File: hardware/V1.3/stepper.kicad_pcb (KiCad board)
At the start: 4 copper layers, 40 x 40 mm, 128 parts, among them J101 USB-MINI-B-SMD, J102 DRILL, J103 DRILL, J104 DRILL, J105 DRILL, J401 STACK-UP-HIGH, J402 STACK-DOWN, J403 STACK-UP-HIGH, J404 STACK-DOWN, P201 black, P202 green, P301 CON-SENSOR, P302 CON-SENSOR, Q201 FDS8449, Q202 AO4421, Q203 2N7002, SW101 Reset, SW102 Erase, U101 AT91SAM3SXB, U102 82400152, U201 ZXCT1086, U202 TMC21XX, U501 LD1117, X101 16Mhz

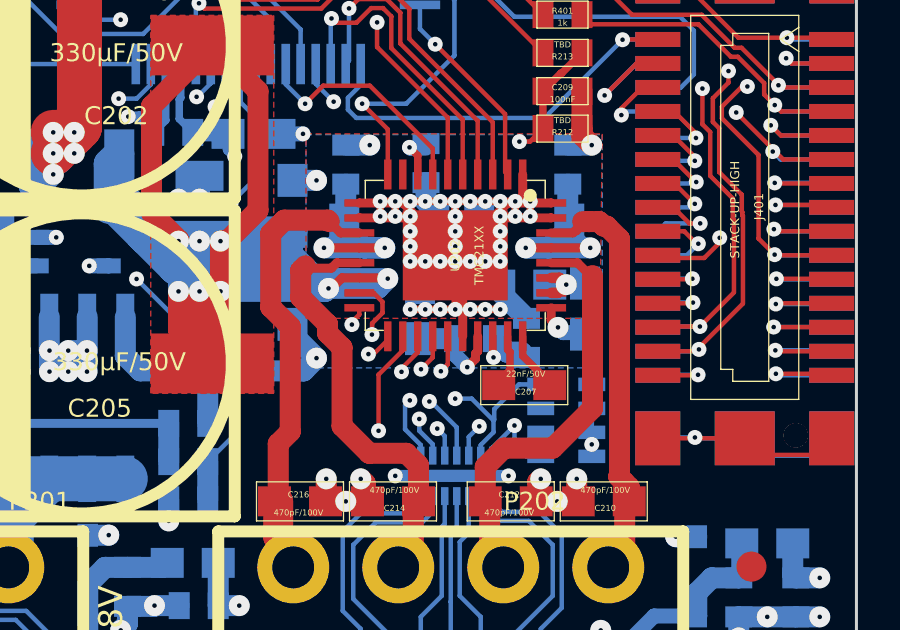
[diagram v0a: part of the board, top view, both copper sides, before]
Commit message: ordered version
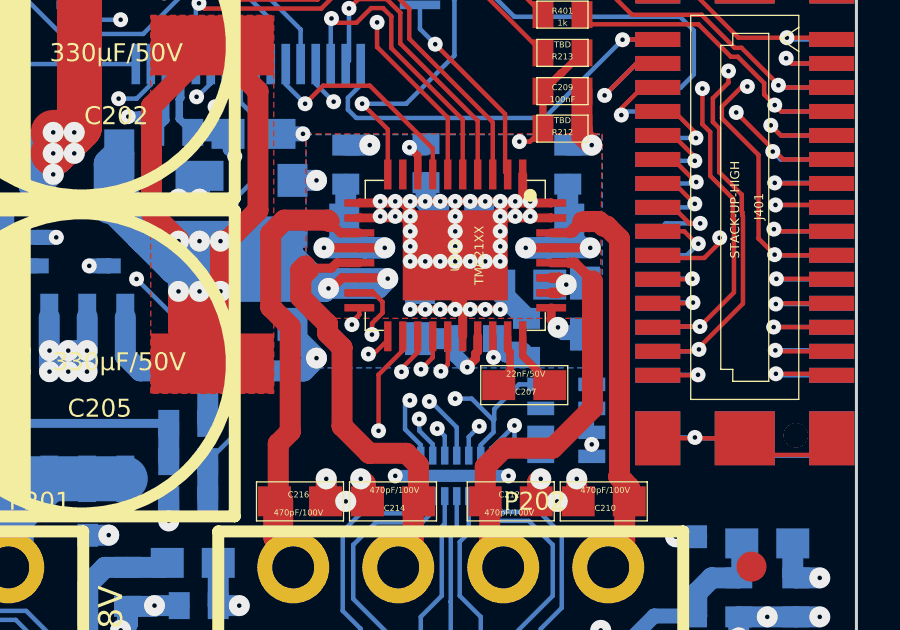
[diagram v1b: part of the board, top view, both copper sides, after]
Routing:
- net M2: track 14.5 -> 15.5 mm
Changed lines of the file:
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@@
     (thickness 1.6002)
     (drawings 64)
-    (tracks 2583)
+    (tracks 2589)
     (zones 0)
     (modules 128)
@@
     (1 GND signal hide)
     (2 VCC signal hide)
-    (31 Rückseite signal hide)
+    (31 Rückseite signal)
     (32 B.Adhes user)
     (33 F.Adhes user)
@@
   )
   (setup
-    (last_trace_width 0.1524)
+    (last_trace_width 0.25)
     (user_trace_width 0.1524)
     (user_trace_width 0.25)
@@
     (pad_to_mask_clearance 0)
     (aux_axis_origin 126.72568 112.776)
-    (visible_elements FFFF5FBF)
+    (visible_elements FFFF9FBF)
     (pcbplotparams
-      (layerselection 0x00030_80000001)
+      (layerselection 0x010f0_80000007)
       (usegerberextensions true)
       (excludeedgelayer true)
       (linewidth 0.150000)
-      (plotframeref true)
+      (plotframeref false)
       (viasonmask false)
       (mode 1)
@@
       (drillshape 0)
       (scaleselection 1)
-      (outputdirectory prod/))
+      (outputdirectory /tmp/stepper/))
   )
   (net 0 "")
@@
   (segment (start 139.15 74.8) (end 139.15 74.3749) (width 0.2998) (layer Rückseite) (net 123))
   (segment (start 139.05 74.6499) (end 139.2 74.8) (width 0.2998) (layer Rückseite) (net 123))
+  (segment (start 157.15 93.6507) (end 157.5257 93.275) (width 0.35) (layer Vorderseite) (net 124))
+  (segment (start 157.6 93.275) (end 157.8 93.275) (width 0.701) (layer Vorderseite) (net 124))
+  (segment (start 157.5257 93.275) (end 157.6 93.275) (width 0.35) (layer Vorderseite) (net 124))
   (segment (start 159.1501 102.6) (end 159.1501 102.1251) (width 0.70104) (layer Vorderseite) (net 124))
   (segment (start 159.1501 102.1251) (end 158.8 101.775) (width 0.70104) (layer Vorderseite) (net 124))
@@
   (segment (start 158.3 93.425) (end 158.3 93.5) (width 0.1524) (layer Vorderseite) (net 124))
   (segment (start 158.3 93.5) (end 158.825 94.025) (width 0.1524) (layer Vorderseite) (net 124))
-  (segment (start 156.54786 93.6507) (end 157.4243 93.6507) (width 0.1524) (layer Vorderseite) (net 124))
-  (segment (start 157.4243 93.6507) (end 157.8 93.275) (width 0.1524) (layer Vorderseite) (net 124))
+  (segment (start 156.54786 93.6507) (end 157.15 93.6507) (width 0.1524) (layer Vorderseite) (net 124))
   (segment (start 158.4 93.425) (end 158.3 93.425) (width 0.701) (layer Vorderseite) (net 124))
   (segment (start 158.15 93.275) (end 157.8 93.275) (width 0.701) (layer Vorderseite) (net 124))
-  (segment (start 157.8 93.275) (end 157.6 93.275) (width 0.701) (layer Vorderseite) (net 124))
   (segment (start 158.3 93.425) (end 158.15 93.275) (width 0.701) (layer Vorderseite) (net 124))
   (segment (start 159 104.25) (end 158.45 104.8) (width 0.701) (layer Vorderseite) (net 124))
@@
   (segment (start 158.4 93.425) (end 158.3 93.425) (width 0.2998) (layer Vorderseite) (net 124))
   (segment (start 158.3 93.425) (end 158.05 93.425) (width 0.2998) (layer Vorderseite) (net 124))
+  (segment (start 157.925 95.25) (end 157.325 94.65) (width 0.35) (layer Vorderseite) (net 125))
+  (segment (start 157.175 94.65) (end 157.175 94.6489) (width 0.35) (layer Vorderseite) (net 125))
+  (segment (start 157.325 94.65) (end 157.175 94.65) (width 0.35) (layer Vorderseite) (net 125))
   (segment (start 154.5 104.35) (end 154.95 104.8) (width 0.701) (layer Vorderseite) (net 125))
   (segment (start 154.5 102.6) (end 154.5 104.35) (width 0.701) (layer Vorderseite) (net 125))
-  (segment (start 157.85 95.075) (end 157.925 95.075) (width 0.2998) (layer Vorderseite) (net 125))
-  (segment (start 157.424 94.6489) (end 157.85 95.075) (width 0.2998) (layer Vorderseite) (net 125))
-  (segment (start 156.548 94.6489) (end 157.424 94.6489) (width 0.2998) (layer Vorderseite) (net 125))
+  (segment (start 156.548 94.6489) (end 157.175 94.6489) (width 0.2998) (layer Vorderseite) (net 125))
   (segment (start 154.35 101.45) (end 154.35 102.425) (width 0.701) (layer Vorderseite) (net 125))
   (segment (start 154.975 100.825) (end 154.35 101.45) (width 0.701) (layer Vorderseite) (net 125))
   (segment (start 156.6 100.825) (end 154.975 100.825) (width 0.701) (layer Vorderseite) (net 125))
   (segment (start 157.925 99.5) (end 156.6 100.825) (width 0.701) (layer Vorderseite) (net 125))
-  (segment (start 157.925 95.075) (end 157.925 99.5) (width 0.701) (layer Vorderseite) (net 125))
+  (segment (start 157.925 95.25) (end 157.925 99.5) (width 0.701) (layer Vorderseite) (net 125))
+  (segment (start 148.2 95.8) (end 148.425 95.575) (width 0.25) (layer Vorderseite) (net 126))
+  (segment (start 148.425 95.225) (end 148.675 94.975) (width 0.25) (layer Vorderseite) (net 126))
+  (segment (start 148.425 95.575) (end 148.425 95.225) (width 0.25) (layer Vorderseite) (net 126))
   (segment (start 149.401 94.6489) (end 150.152 94.6489) (width 0.2998) (layer Vorderseite) (net 126))
   (segment (start 149.225 94.825) (end 149.401 94.6489) (width 0.2998) (layer Vorderseite) (net 126))
@@
   (segment (start 149.0916 96.9881) (end 149.5764 97.4729) (width 0.701) (layer Vorderseite) (net 126))
   (segment (start 149.0916 96.6916) (end 149.0916 96.9881) (width 0.701) (layer Vorderseite) (net 126))
+  (segment (start 148.2 95.8) (end 148.2 95.8) (width 0.701) (layer Vorderseite) (net 126))
   (segment (start 148.2 95.8) (end 149.0916 96.6916) (width 0.701) (layer Vorderseite) (net 126))
   (segment (start 148.2 94.9) (end 148.2 95.8) (width 0.701) (layer Vorderseite) (net 126))
